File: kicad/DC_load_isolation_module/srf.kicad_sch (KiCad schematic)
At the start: 43 parts, among them Q1 MMBT5551L, Q26 MMBT5551L, Q27 MMBT5551L, Q28 MMBT5551L, Q29 MMBT5551L, T2 UMEC_UT20A13S

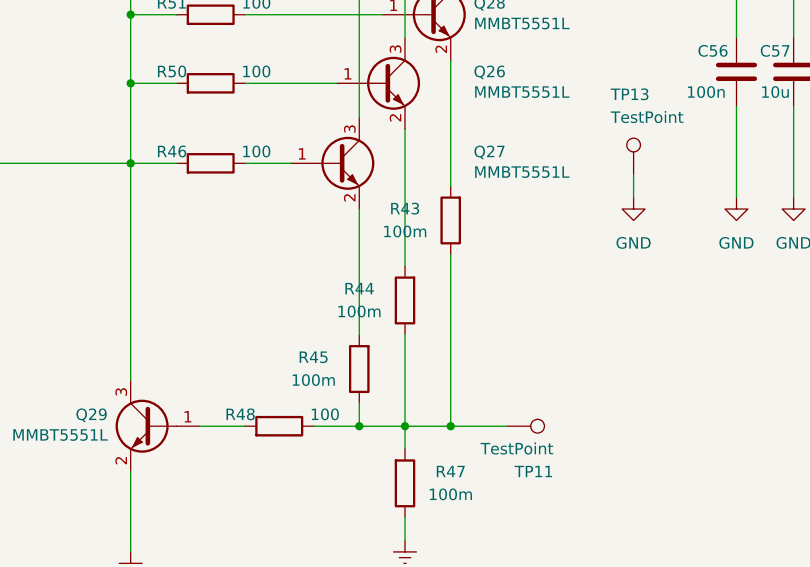
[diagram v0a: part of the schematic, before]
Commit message: kfsald
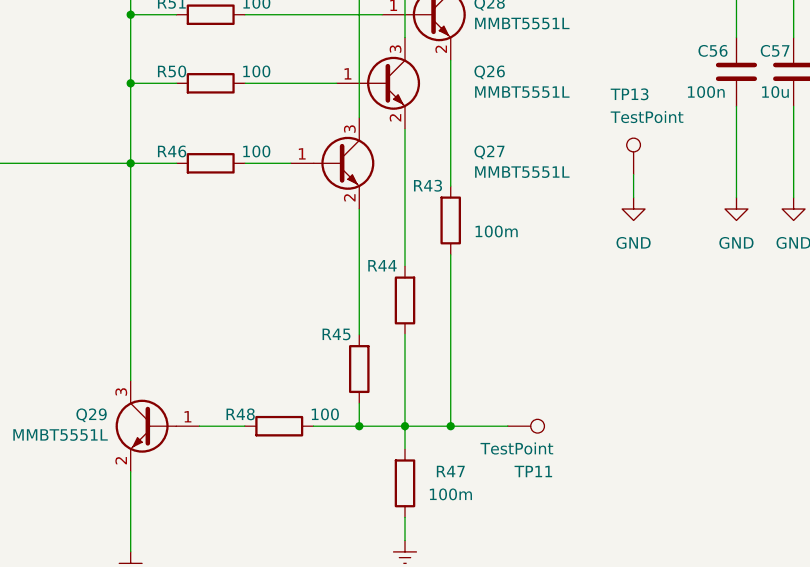
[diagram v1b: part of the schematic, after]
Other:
- moved on the sheet: R43
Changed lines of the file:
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@@
 	(symbol
 		(lib_id "Device:R")
-		(at 95.25 140.97 180)
+		(at 95.25 140.97 0)
+		(mirror x)
 		(unit 1)
 		(exclude_from_sim no)
@@
 		(dnp no)
 		(property "Reference" "R43"
-			(at 90.17 139.7 0)
+			(at 92.71 137.16 0)
 			(effects
 				(font
@@
 		)
 		(property "Value" "100m"
-			(at 90.17 142.24 0)
+			(at 100.33 142.24 0)
 			(effects
 				(font
@@
 		)
 		(property "Footprint" "Resistor_SMD:R_1206_3216Metric_Pad1.30x1.75mm_HandSolder"
-			(at 97.028 140.97 90)
+			(at 93.472 140.97 90)
 			(effects
 				(font
@@
 		(dnp no)
 		(property "Reference" "R44"
-			(at 85.09 148.59 0)
+			(at 87.63 146.05 0)
 			(effects
 				(font
@@
 		)
 		(property "Value" "100m"
-			(at 85.09 151.13 0)
-			(effects
-				(font
-					(size 1.27 1.27)
-				)
+			(at 87.63 152.4 0)
+			(effects
+				(font
+					(size 1.27 1.27)
+				)
+				(hide yes)
 			)
 		)
@@
 		(dnp no)
 		(property "Reference" "R45"
-			(at 80.01 156.21 0)
+			(at 82.55 153.67 0)
 			(effects
 				(font
@@
 		)
 		(property "Value" "100m"
-			(at 80.01 158.75 0)
-			(effects
-				(font
-					(size 1.27 1.27)
-				)
-			)
-		)
+			(at 81.28 157.48 0)
+			(effects
+				(font
+					(size 1.27 1.27)
+				)
+				(hide yes)
+			)
+		)
